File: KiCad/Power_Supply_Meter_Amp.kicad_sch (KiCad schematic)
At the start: 630 parts, among them J1 R_Phono_In, J10 VCC_IN, J11 VCC_OUT, J12 EMK_In, J13 EMK_Out, J14 EMK_Out, J15 Mic_Effekt_Out, J16 Mic_Effekt_Out, J17 Mic_Effekt_Out, J18 Mic_Effekt_Out, J19 Phono/Line_Out, J2 L_Phono_In, J20 Mic_Effekt_Out, J21 Conn_01x05_bridged, J22 EMK_In, J24 Mic_Effekt_In, J25 Mic_Effekt_In, J26 Phono/Line_In, J27 Mic_Effekt_In, J28 Pegel_Out, J29 Pegel_Out, J3 R_Line_In, J30 Pegel_In, J31 Pegel_In, J32 Pegel_In, J33 Pegel_In, J34 LED_Out, J35 LED_In, J36 VU_Meter_Out, J37 AUX_Send_3, J38 AUX_Send_1, J39 AUX_Send_2, J4 L_Line_In, J40 Bass_Out, J41 Kick_Out, J42 Mid_Out, J43 High_Out, J44 Line_Out_L, J45 Line_Out_R, J5 Mic_In, J6 Effekt_In, J7 AUX_RET_1, J8 AUX_RET_2, J9 AUX_RET_3, SW1 SW_DPST, SW10 SW_SPDT, SW11 SW_SPDT, SW12 SW_SPDT, SW2 SW_SPDT, SW3 SW_SPDT, SW4 SW_SPDT, SW5 SW_SPDT, SW6 SW_SPDT, SW7 SW_SPDT, SW8 SW_SPDT, SW9 SW_Rotary_1x4, U1 TL074, U10 TL074, U11 TL074, U12 TL074, U13 TL074, U14 TL074, U15 TL074, U16 TL074, U17 TL074, U18 TL074, U19 TL074, U2 TL074, U20 TL074, U21 TL074, U22 TL074, U23 TL074, U24 TL074, U25 INA128U, U3 TL074, U4 TL074, U5 TL074, U6 REC10K-2409, U7 REC10K-2415, U8 TL074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

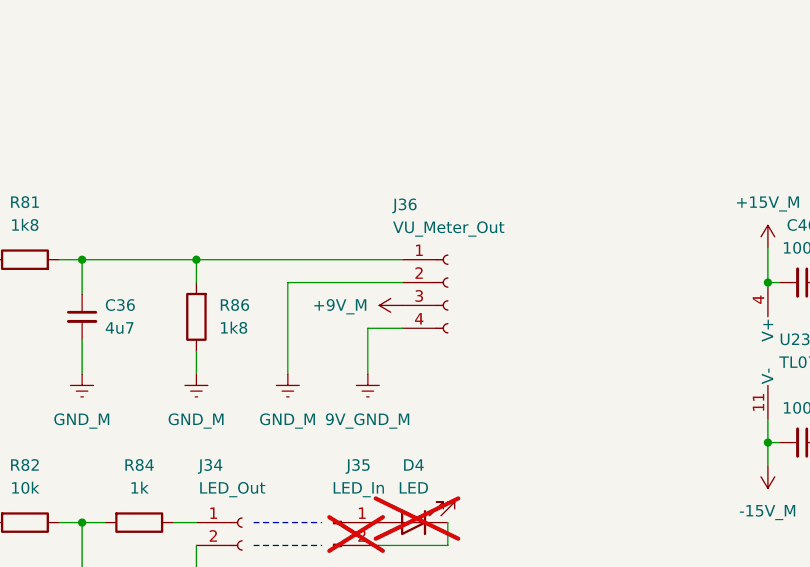
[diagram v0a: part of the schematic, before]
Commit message: PCB Update
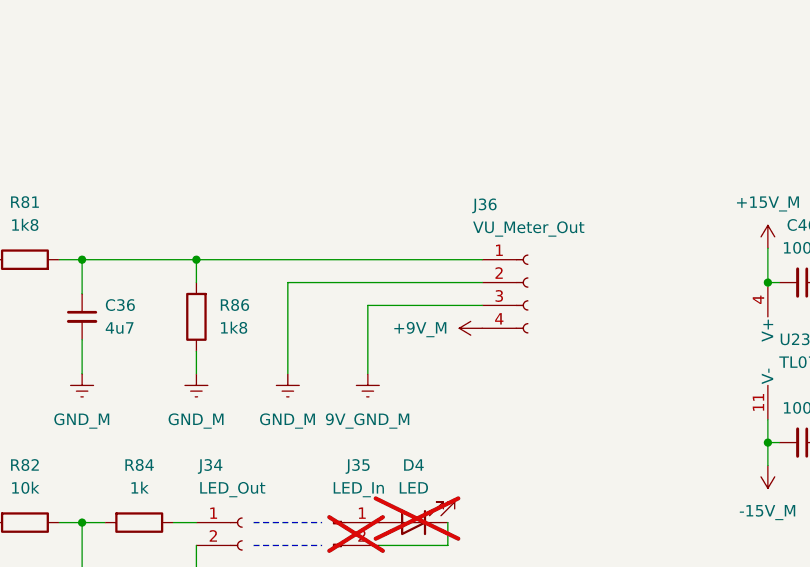
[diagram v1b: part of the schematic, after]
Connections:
- net +9V_M: now also J36.4 (Pin_4); no longer J36.3 (Pin_3)
- net 9V_GND_M: now also J36.3 (Pin_3); no longer J36.4 (Pin_4)
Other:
- moved on the sheet: J36
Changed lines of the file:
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@@
 	(wire
 		(pts
-			(xy 637.54 525.78) (xy 637.54 520.7)
+			(xy 637.54 518.16) (xy 637.54 525.78)
 		)
 		(stroke
@@
 	(wire
 		(pts
-			(xy 637.54 520.7) (xy 641.35 520.7)
-		)
-		(stroke
-			(width 0)
-			(type default)
-		)
-	)
-	(wire
-		(pts
 			(xy 368.3 238.76) (xy 365.76 238.76)
 		)
@@
 	(wire
 		(pts
+			(xy 637.54 518.16) (xy 650.24 518.16)
+		)
+		(stroke
+			(width 0)
+			(type default)
+		)
+	)
+	(wire
+		(pts
 			(xy 487.68 283.21) (xy 490.22 283.21)
 		)
@@
 	(wire
 		(pts
-			(xy 618.49 513.08) (xy 641.35 513.08)
+			(xy 618.49 513.08) (xy 650.24 513.08)
 		)
 		(stroke
@@
 	(wire
 		(pts
-			(xy 628.65 515.62) (xy 641.35 515.62)
+			(xy 628.65 515.62) (xy 650.24 515.62)
 		)
 		(stroke
@@
 	(symbol
 		(lib_id "Connector:Conn_01x04_Socket")
-		(at 646.43 515.62 0)
+		(at 655.32 515.62 0)
 		(unit 1)
 		(exclude_from_sim no)
@@
 		(dnp no)
 		(property "Reference" "J36"
-			(at 640.334 506.984 0)
+			(at 649.224 506.984 0)
 			(effects
 				(font
@@
 		)
 		(property "Value" "VU_Meter_Out"
-			(at 640.334 509.524 0)
+			(at 649.224 509.524 0)
 			(effects
 				(font
@@
 		)
 		(property "Footprint" "Connector_PinSocket_2.54mm_LongPads:PinSocket_1x04_P2.54mm_Vertical_LongPdas"
-			(at 646.43 515.62 0)
+			(at 655.32 515.62 0)
 			(effects
 				(font
@@
 		)
 		(property "Datasheet" "~"
-			(at 646.43 515.62 0)
+			(at 655.32 515.62 0)
 			(effects
 				(font
@@
 		)
 		(property "Description" "Generic connector, single row, 01x04, script generated"
-			(at 646.43 515.62 0)
+			(at 655.32 515.62 0)
 			(effects
 				(font
@@
 	(symbol
 		(lib_id "power:VCC")
-		(at 641.35 518.16 90)
+		(at 650.24 520.7 90)
 		(unit 1)
 		(exclude_from_sim no)
@@
 		(fields_autoplaced yes)
 		(property "Reference" "#PWR0197"
-			(at 645.16 518.16 0)
+			(at 654.05 520.7 0)
 			(effects
 				(font
@@
 		)
 		(property "Value" "+9V_M"
-			(at 637.54 518.1599 90)
+			(at 646.43 520.6999 90)
 			(effects
 				(font
@@
 		)
 		(property "Footprint" ""
-			(at 641.35 518.16 0)
+			(at 650.24 520.7 0)
 			(effects
 				(font
@@
 		)
 		(property "Datasheet" ""
-			(at 641.35 518.16 0)
+			(at 650.24 520.7 0)
 			(effects
 				(font
@@
 		)
 		(property "Description" "Power symbol creates a global label with name \"VCC\""
-			(at 641.35 518.16 0)
+			(at 650.24 520.7 0)
 			(effects
 				(font
